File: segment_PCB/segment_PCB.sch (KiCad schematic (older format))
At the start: 36 parts, among them J2 #AVR-ISP-6, SW1 SW_Push, U4 74HC138, Y1 12MHz

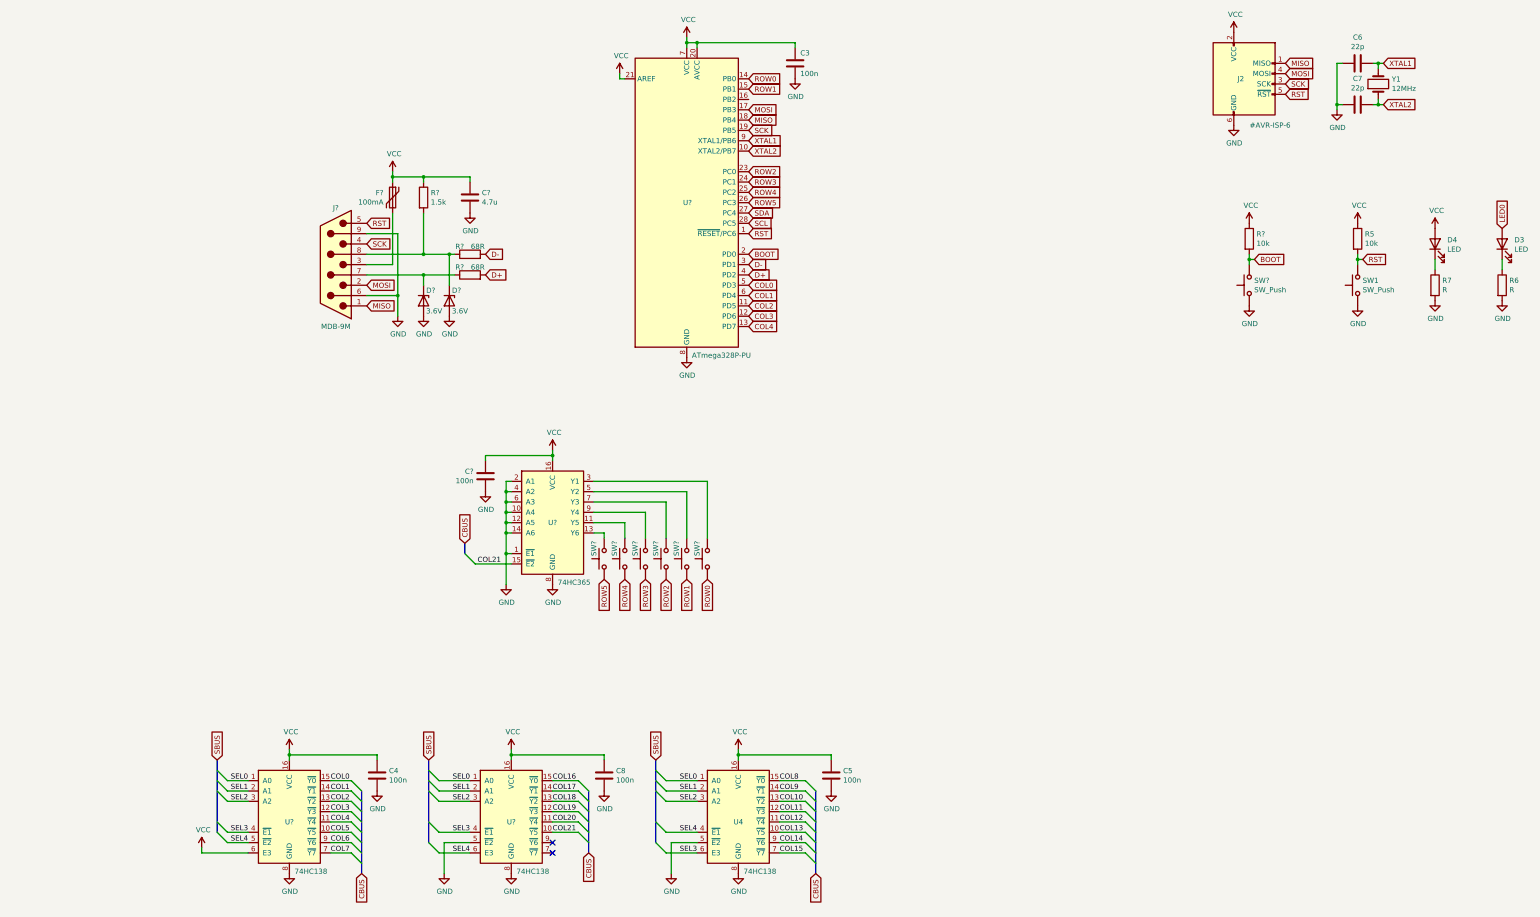
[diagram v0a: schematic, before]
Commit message: Started mock keyboard
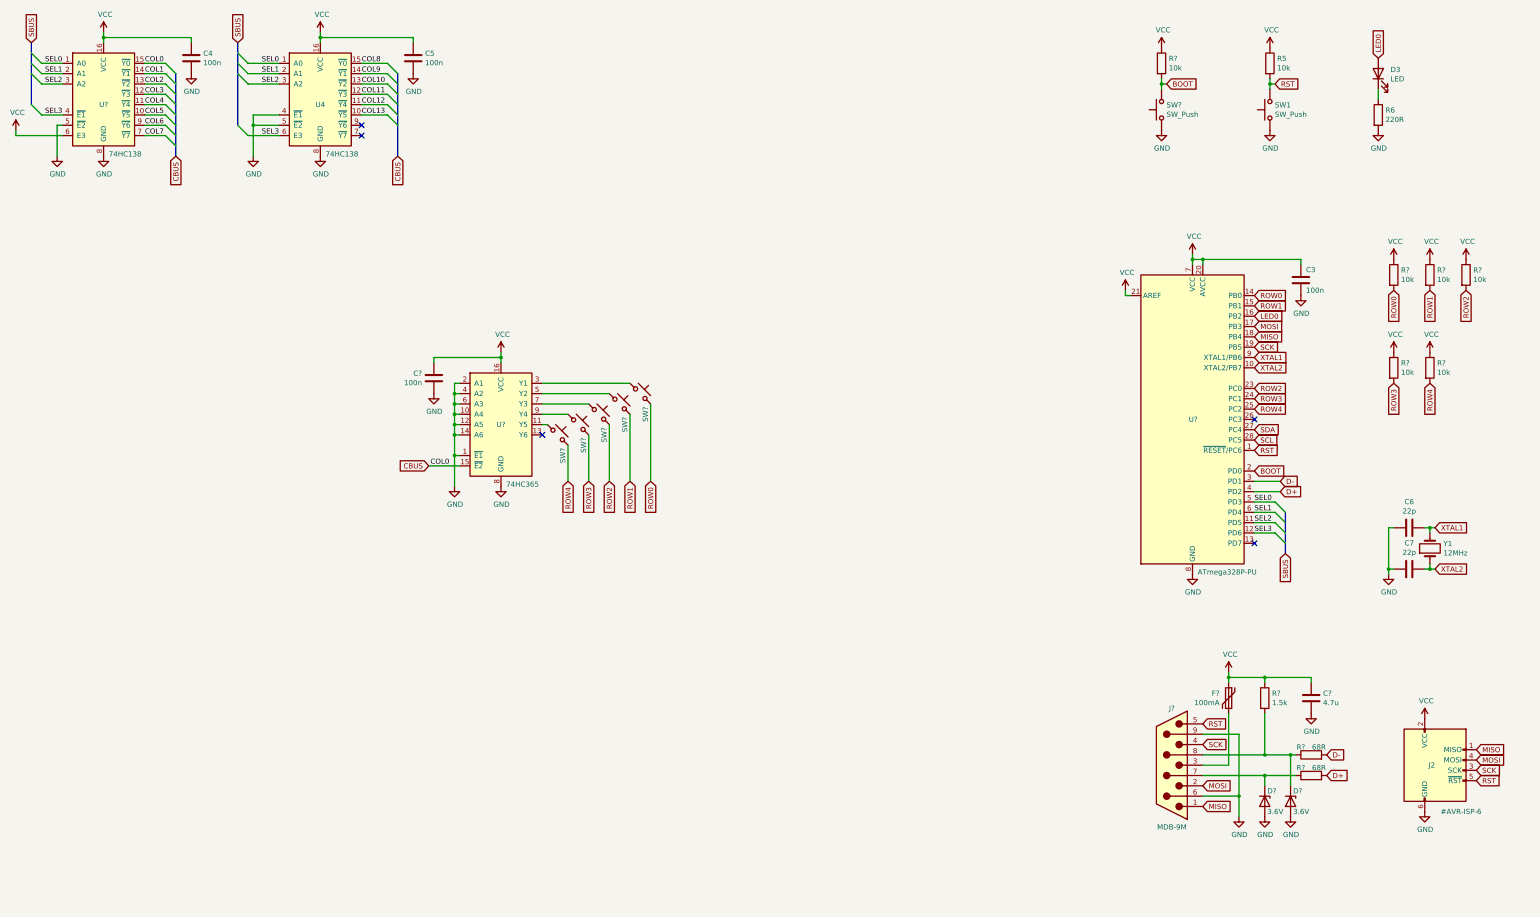
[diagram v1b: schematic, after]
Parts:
- removed C8, C?: 100n, Capacitor_THT:C_Disc_D3.0mm_W1.6mm_P2.50mm, symbol Device:C
- removed D4: LED, LED_THT:LED_D5.0mm, symbol Device:LED
- removed R7: R, Resistor_THT:R_Axial_DIN0204_L3.6mm_D1.6mm_P5.08mm_Horizontal, symbol Device:R
- removed SW? (x6): SW_Push, symbol Switch:SW_Push
- removed U?: 74HC138, symbol Segment_Parts:74HC138
- removed U?: 74HC365, symbol Segment_Parts:74HC365
- added C?: 100n, Capacitor_THT:C_Disc_D3.0mm_W1.6mm_P2.50mm, symbol Device:C
- added R? (x5): 10k, symbol Device:R
- added SW? (x5): SW_Push_45deg, symbol Switch:SW_Push_45deg
- added U?: 74HC365, symbol Segment_Parts:74HC365
- R6: value R -> 220R
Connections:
- net SEL4 is gone; now on net GND: U4.4 (~E1), U?.5 (~E2)
- net CBUS: now also U?.15 (~Y0), U?.15 (~E2)
- net COL1: no longer U?.6 (PD4)
- net COL2: no longer U?.11 (PD5)
- net COL3: no longer U?.12 (PD6)
- net COL4: no longer U?.13 (PD7)
- net GND: now also C?.2, U?.1 (~E1), U?.10 (A4), U?.12 (A5), U?.14 (A6), U?.2 (A1), U?.4 (A2), U?.6 (A3), U?.8 (GND)
- net LED0: now also U?.16 (PB2)
- net ROW0: now also R?.2, SW?.2
- net ROW1: now also R?.2, SW?.2
- net ROW2: now also R?.2, SW?.2
- net ROW3: now also R?.2, SW?.2
- net ROW4: now also R?.2, SW?.2
- net SEL0: now also U?.5 (PD3)
- net SEL1: now also U?.6 (PD4)
- net SEL2: now also U?.11 (PD5)
- net SEL3: now also U?.12 (PD6)
- net VCC: now also C?.1, R?.1, R?.1, R?.1, R?.1, R?.1, U?.16 (VCC)
- removed net COL0: U?.15 (~Y0), U?.5 (PD3)
- net COL14: no longer names the net of U4.9 (~Y6)
- net COL15: no longer names the net of U4.7 (~Y7)
- net ROW5: no longer names the net of U?.26 (PC3)
- new net: SW?.1, U?.11 (Y5)
- new net: SW?.1, U?.3 (Y1)
- new net: SW?.1, U?.5 (Y2)
- new net: SW?.1, U?.7 (Y3)
- new net: SW?.1, U?.9 (Y4)
- no-connect marks 2 -> 5
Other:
- moved on the sheet: C3, C4, C5, C6, C7, C?, D3, D?, F?, J2, J?, R5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
